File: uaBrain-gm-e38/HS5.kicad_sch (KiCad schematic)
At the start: 30 parts, among them U5 BSP762TXUMA1, U6 BSP762TXUMA1, U7 BSP762TXUMA1, U8 BSP762TXUMA1, U9 BSP762TXUMA1

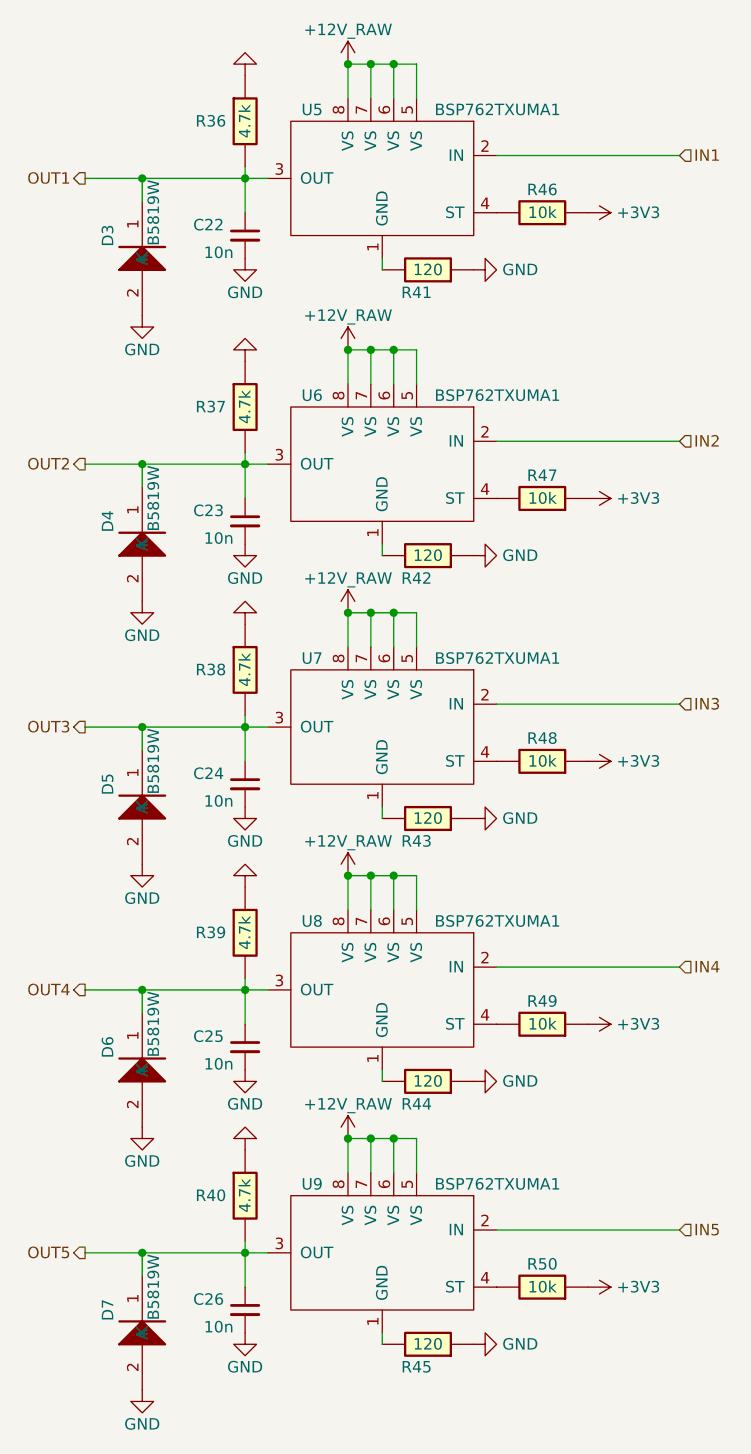
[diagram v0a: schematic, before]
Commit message: uaBrain-e38 rev a
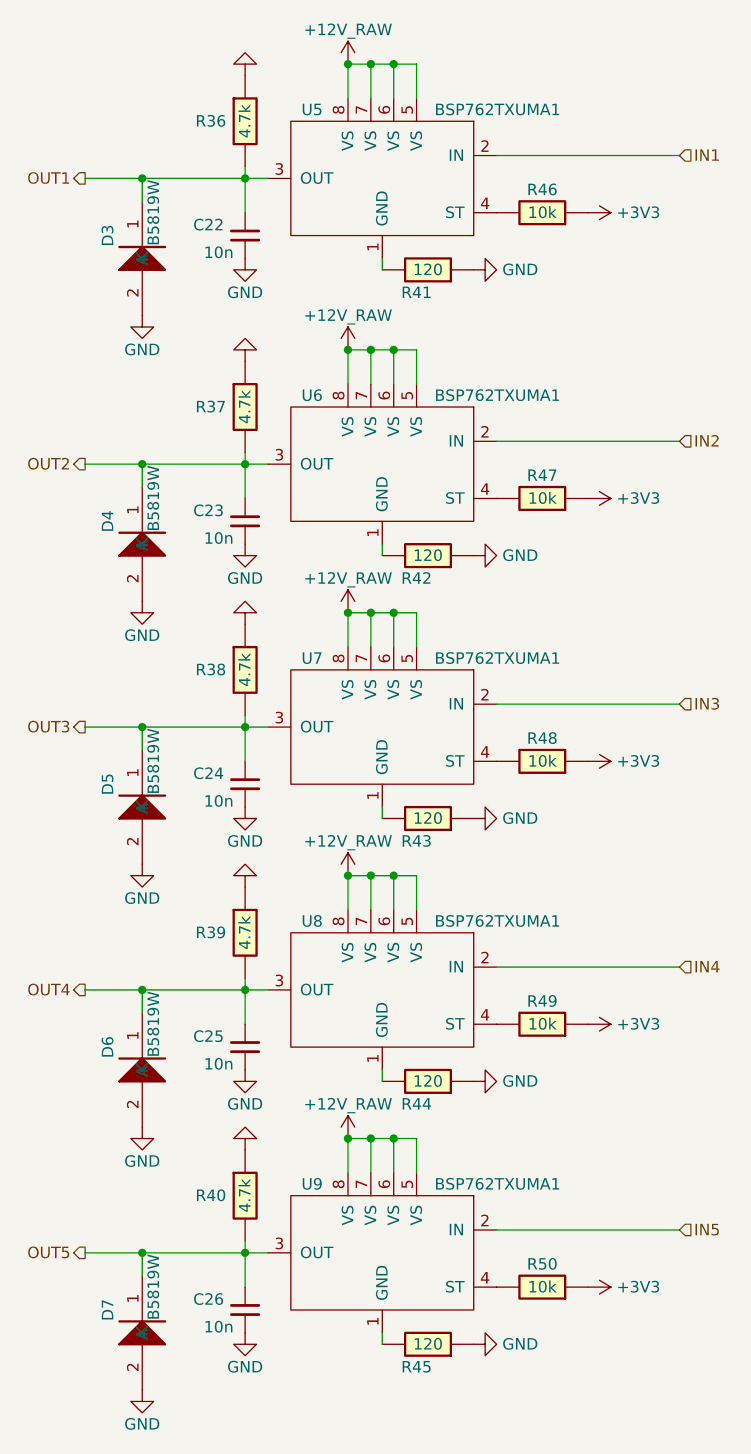
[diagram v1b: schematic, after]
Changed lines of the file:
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@@
 			)
 		)
-		(property "Description" ""
+		(property "Description" "Unpolarized capacitor, small symbol"
 			(at 115.57 156.21 0)
 			(hide yes)
@@
 			)
 		)
-		(property "Description" ""
+		(property "Description" "Unpolarized capacitor, small symbol"
 			(at 115.57 36.83 0)
 			(hide yes)
@@
 			)
 		)
-		(property "Description" ""
+		(property "Description" "Unpolarized capacitor, small symbol"
 			(at 115.57 127 0)
 			(hide yes)
@@
 			)
 		)
-		(property "Description" ""
+		(property "Description" "Unpolarized capacitor, small symbol"
 			(at 115.57 68.58 0)
 			(hide yes)
@@
 			)
 		)
-		(property "Description" ""
+		(property "Description" "Unpolarized capacitor, small symbol"
 			(at 115.57 97.79 0)
 			(hide yes)
